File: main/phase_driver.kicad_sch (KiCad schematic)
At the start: 7 parts, among them Q401 TK4R3E06PL, Q402 TK4R3E06PL

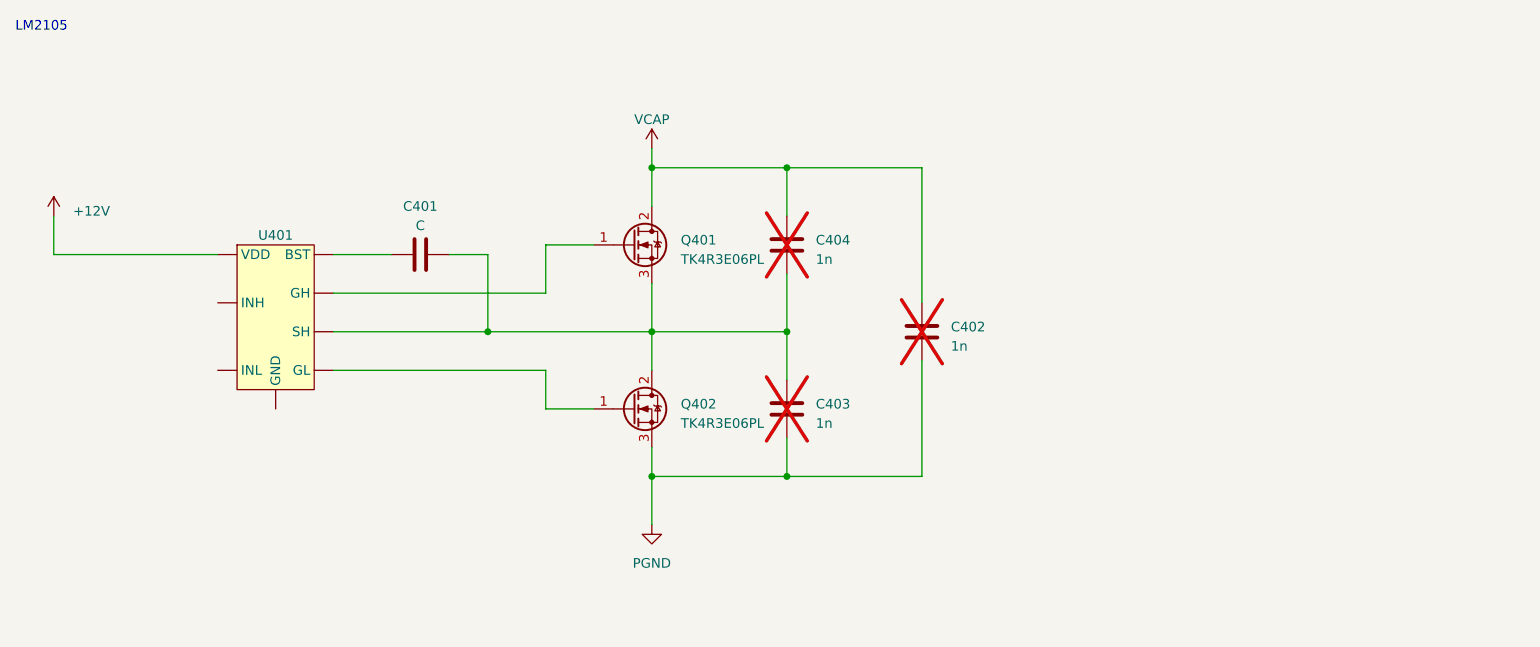
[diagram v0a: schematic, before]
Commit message: PSU should be OK
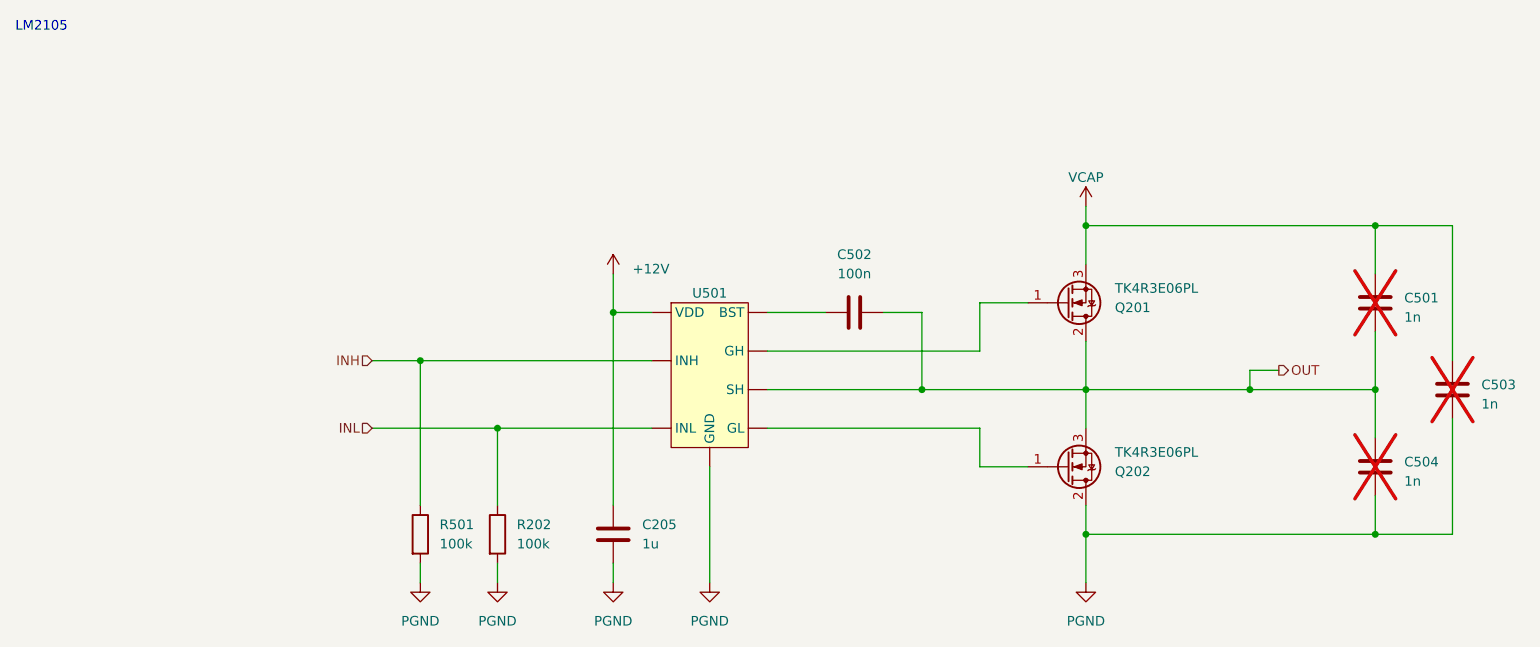
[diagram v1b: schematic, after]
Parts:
- removed Q401, Q402: TK4R3E06PL, Package_TO_SOT_THT:TO-220-3_Horizontal_TabUp, symbol Device:Q_NMOS_GDS
- added C205: 1u, symbol Device:C
- added Q201, Q202: TK4R3E06PL, Package_TO_SOT_THT:TO-220-3_Horizontal_TabUp, symbol Device:Q_NMOS_GDS
- added R202, R501: 100k, symbol Device:R
- C502: renamed from C401; value C -> 100n
- renumbered C404 to C501, C402 to C503, C403 to C504, U401 to U501
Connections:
- net +12V: now also C205.1
- net PGND: now also U501. (VDD), C205.2, Q202.2 (D), R202.2, R501.2
- net VCAP: now also Q201.3 (S)
- net OUT: now reaches C501.2, C502.2, C504.1, U501. (VDD)
- net OUT: now also Q201.2 (D), Q202.3 (S)
- new net: Q202.1 (G), U501. (VDD)
- new net: Q201.1 (G), U501. (VDD)
- new net INH: R501.1, U501. (VDD)
- new net INL: R202.1, U501. (VDD)
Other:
- moved on the sheet: C501, C502, C503, C504, U501
